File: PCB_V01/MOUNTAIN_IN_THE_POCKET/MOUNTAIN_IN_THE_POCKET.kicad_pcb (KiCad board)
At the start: 2 copper layers, 1 part, among them U1 AS1115-BSST

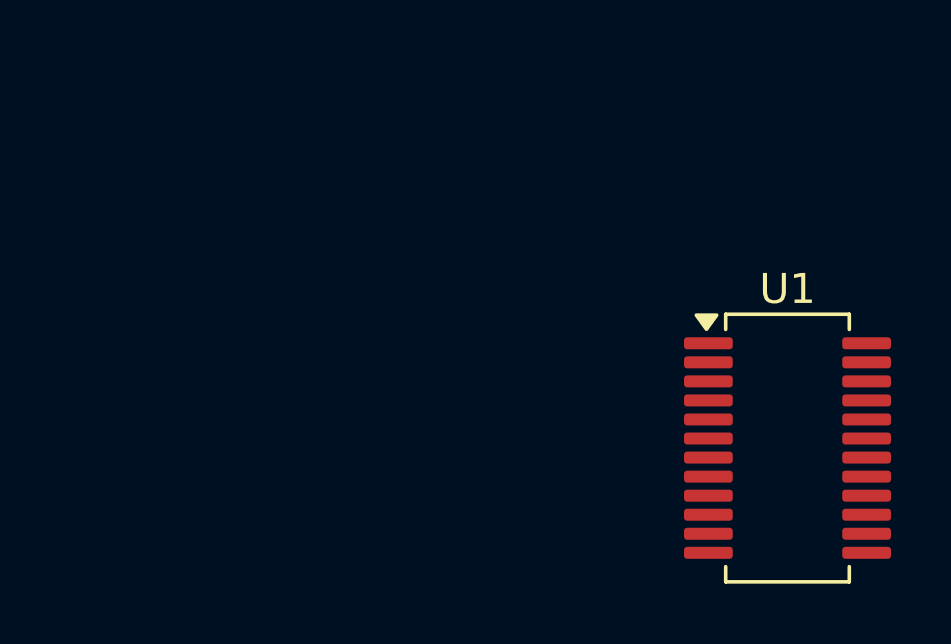
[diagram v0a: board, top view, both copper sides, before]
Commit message: SCH en proceso
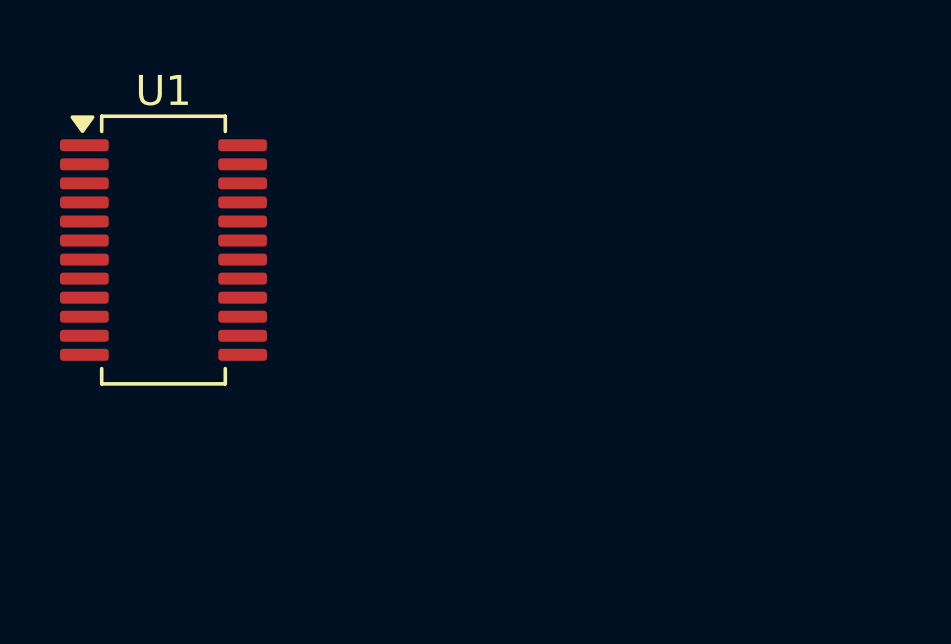
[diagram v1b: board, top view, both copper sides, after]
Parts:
- moved U1 21.8 mm to (33.1, 33.0)
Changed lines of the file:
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@@
 	(footprint "Package_SO:QSOP-24_3.9x8.7mm_P0.635mm"
 		(layer "F.Cu")
-		(at 53.925 39.625)
+		(at 33.125 33.025)
 		(descr "QSOP, 24 Pin (https://pdfserv.maximintegrated.com/package_dwgs/21-0055.PDF)")
 		(tags "QSOP SO")
